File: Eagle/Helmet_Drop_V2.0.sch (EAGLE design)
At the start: 30 parts, among them Q3 MOSFET-NCH, Q4 MOSFET-NCH, Q5 MOSFET-NCH, U1 TH_DS_LIBRARIES_ITSYBITSY_5V, X1 MSTBA4, X2 TH_DS_LIBRARIES_MSTBA4

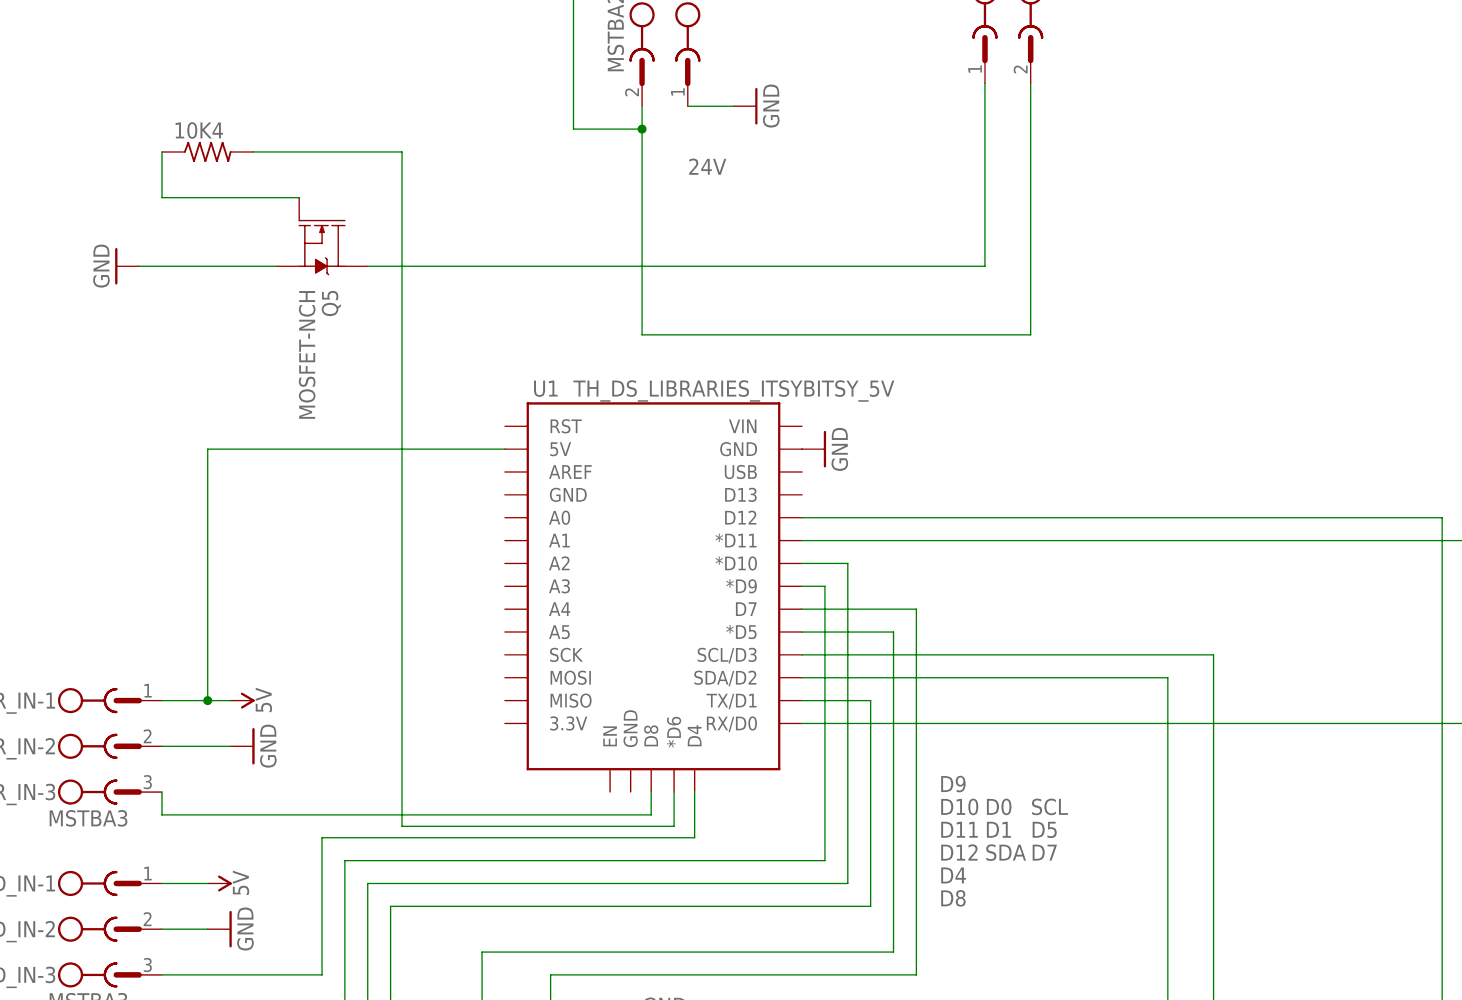
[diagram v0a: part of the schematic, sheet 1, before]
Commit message: update
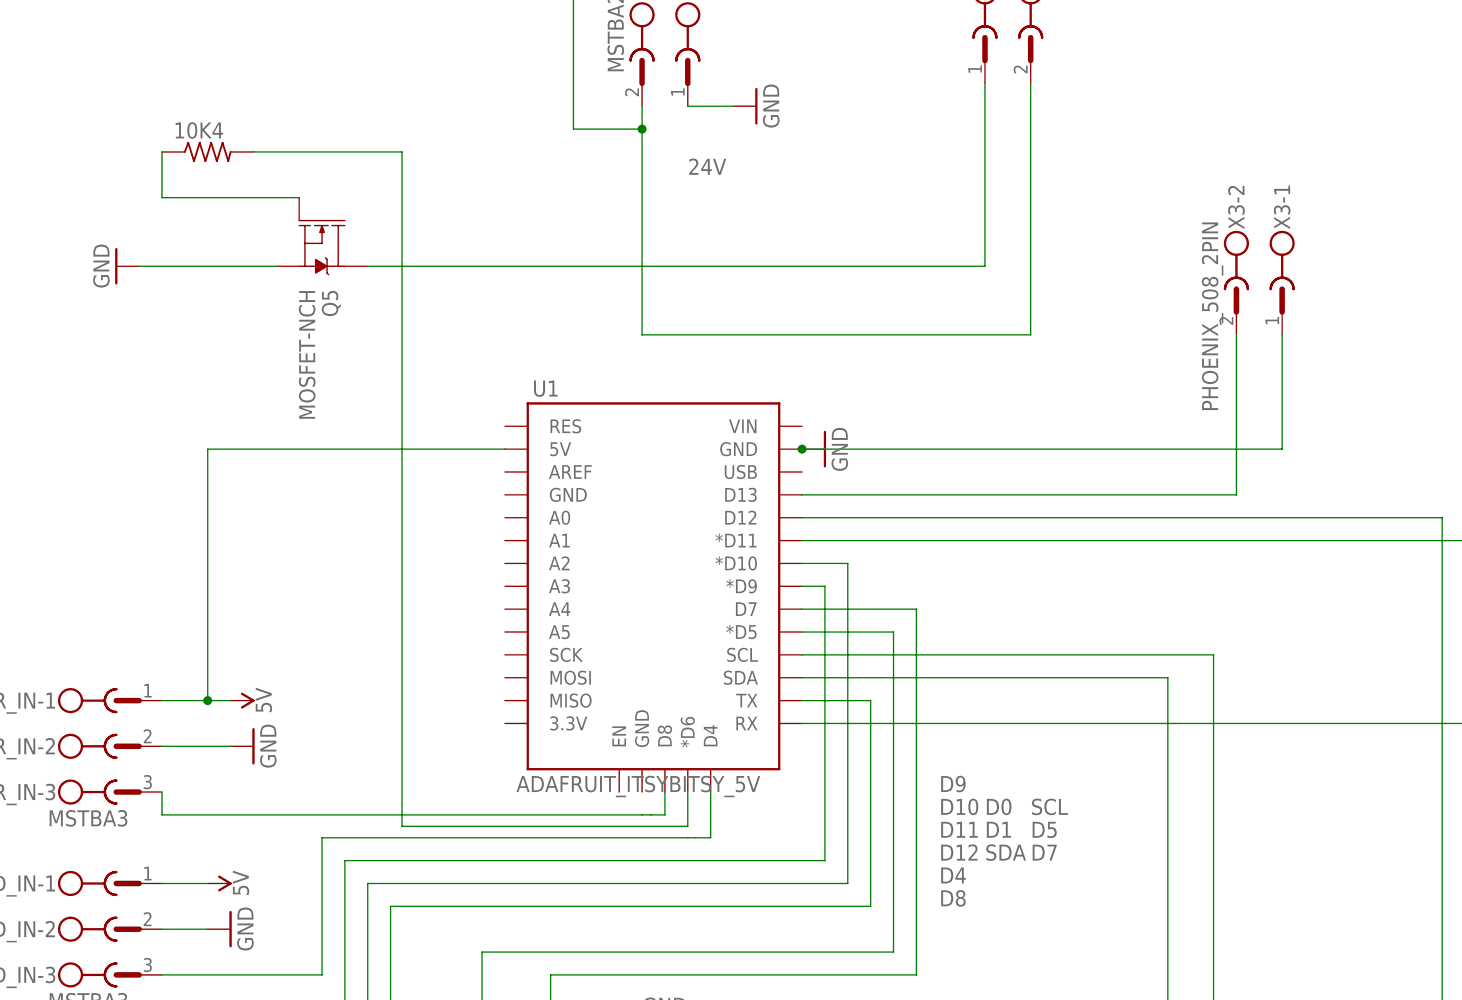
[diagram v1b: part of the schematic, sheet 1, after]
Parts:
- added X3: PHOENIX_508_2PIN, OMSI_Default_V1:PHOENIX_508_2PIN
- U1: value TH_DS_LIBRARIES_ITSYBITSY_5V -> ADAFRUIT_ITSYBITSY_5V; device Helmet_Drop_V1.5:TH_DS_LIBRARIES_ITSYBITSY_5V -> OMSI_Default_V1:ADAFRUIT_ITSYBITSY_5V
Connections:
- new net N$2: U1.D13, X3-2.1
- net D0: now also U1.RX; no longer U1.RX/D0
- net D1: now also U1.TX; no longer U1.TX/D1
- net GND: now also X3-1.1
- net SCL: now also U1.SCL; no longer U1.SCL/D3
- net SDA: now also U1.SDA; no longer U1.SDA/D2
